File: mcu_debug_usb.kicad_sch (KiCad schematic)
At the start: 9 parts, among them IC3 ESDALC6V1W5, J1 USB4105-GF-A

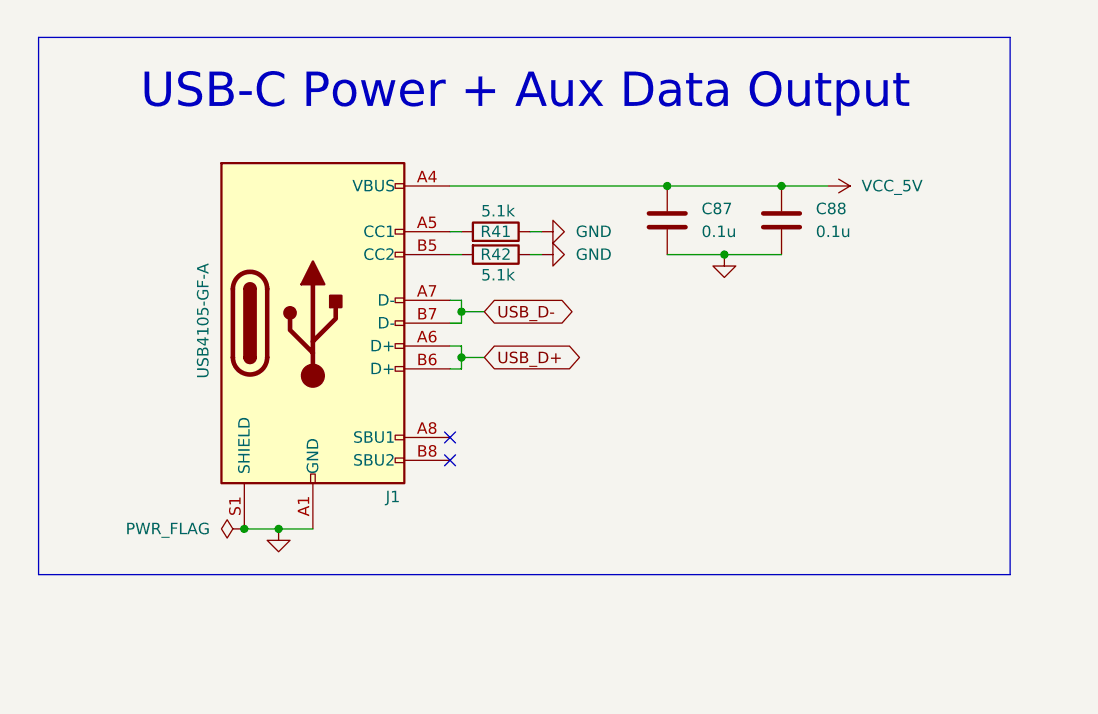
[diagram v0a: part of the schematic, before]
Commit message: Updates for Rev. C
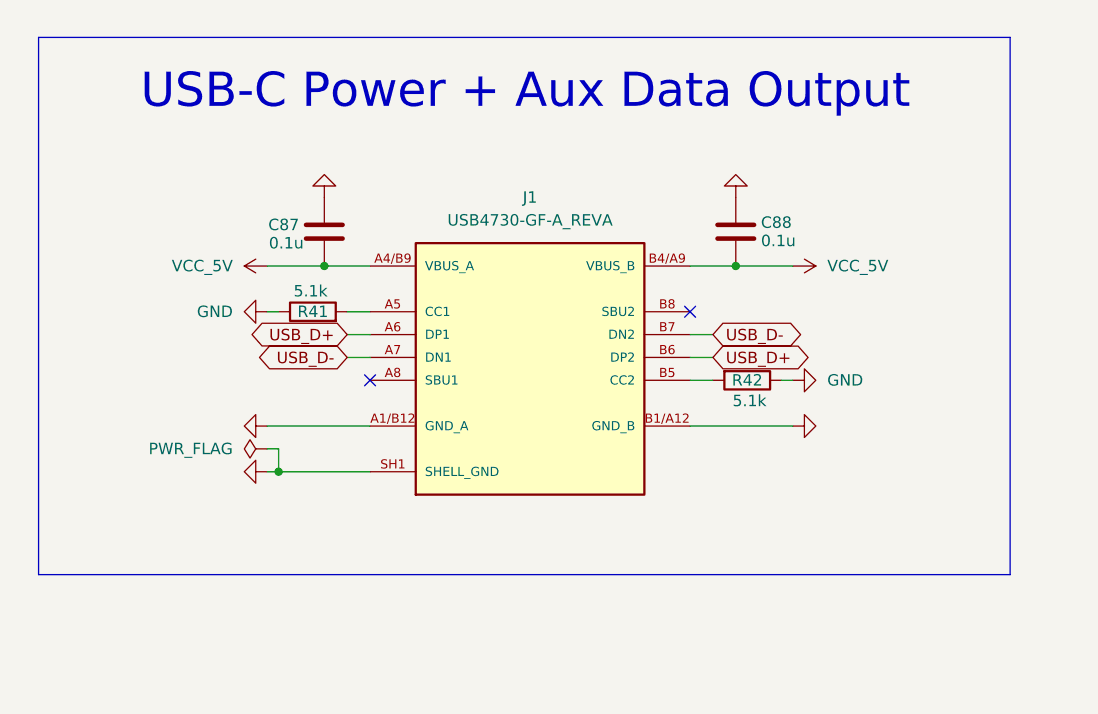
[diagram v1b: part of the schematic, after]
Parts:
- removed J1: USB4105-GF-A, Connector_USB:USB_C_Receptacle_GCT_USB4105-xx-A_16P_TopMnt_Horizontal, symbol Connector:USB_C_Receptacle_USB2.0_16P
- added J1: USB4730-GF-A_REVA, CivicAlert:USB4730-GF-A, symbol USB4730-GF-A:USB4730-GF-A_REVA
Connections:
- net GND: now also J1.A1/B12 (GND_A), J1.B1/A12 (GND_B), J1.SH1 (SHELL_GND), J1.SH2 (SHELL_GND), J1.SH3 (SHELL_GND), J1.SH4 (SHELL_GND)
- net USB_D+: now also J1.A6 (DP1), J1.B6 (DP2)
- net USB_D-: now also J1.A7 (DN1), J1.B7 (DN2)
- net VCC_5V: now also J1.A4/B9 (VBUS_A), J1.B4/A9 (VBUS_B)
- net at R42.2: now also J1.B5 (CC2)
- net at R41.2: now also J1.A5 (CC1)
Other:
- moved on the sheet: C87, C88, R41, R42
